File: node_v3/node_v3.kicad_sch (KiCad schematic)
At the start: 61 parts, among them J1 Conn_Coaxial, J10 3V3OUT, J12 12402012E212A, J13 DBG, J14 VIN, J15 Conn_01x16_Pin, J2 Micro_SD_Card, J6 BAT, Q1 2N3904, SW1 PTS526, SW2 PTS526, U1 RFM69HCW, U2 MCP7940N-xSN, U3 MCP73831-2-OT, U4 ADP2108AUJ-3.3, U5 CAT3200-5, U6 RP2040, U7 W25Q128JVS, Y1 445C35A12M00000, Y2 SC32S-7PF20PPM

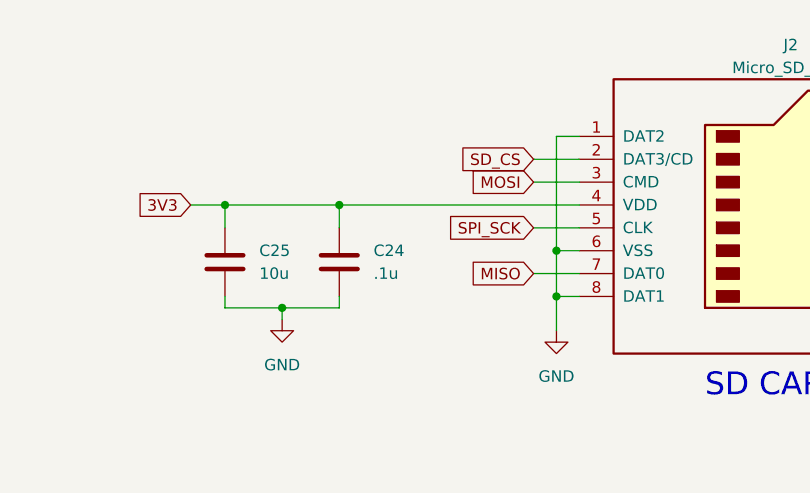
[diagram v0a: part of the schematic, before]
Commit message: not finished yet
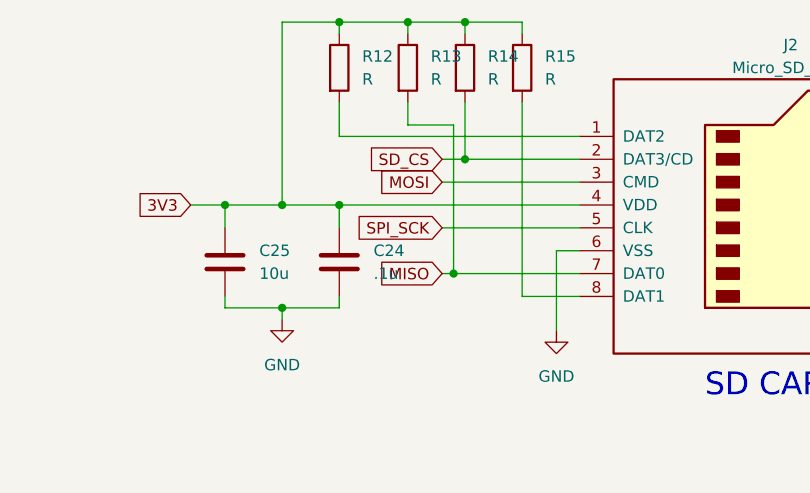
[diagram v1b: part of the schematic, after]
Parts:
- added R12, R13, R14, R15: R, Resistor_SMD:R_0805_2012Metric_Pad1.20x1.40mm_HandSolder, symbol Device:R
- U1: footprint RF_Module:HOPERF_RFM69HW -> custom:HOPERF_RFM9XW_SMD
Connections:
- net 3V3: now also R12.1, R13.1, R14.1, R15.1
- net GND: no longer J2.1 (DAT2), J2.8 (DAT1)
- net MISO: now also R13.2
- net SD_CS: now also R14.2
- new net: J2.1 (DAT2), R12.2
- new net: J2.8 (DAT1), R15.2
